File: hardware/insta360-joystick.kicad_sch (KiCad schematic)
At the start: 12 parts

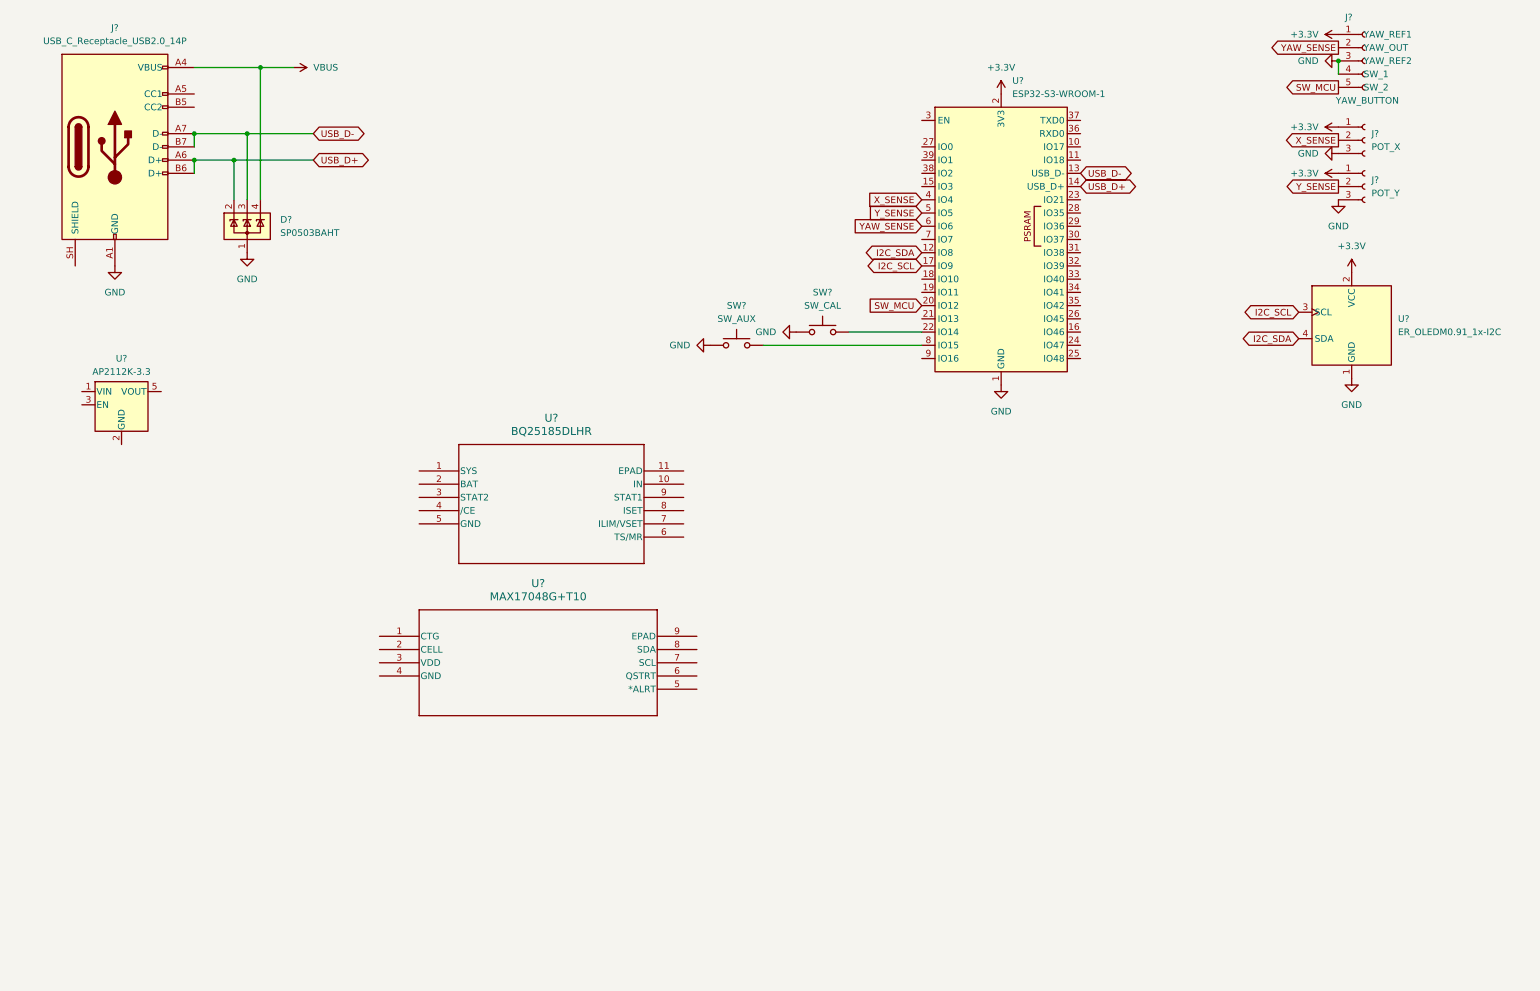
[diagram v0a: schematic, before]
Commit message: Ok I think the schematic is done?
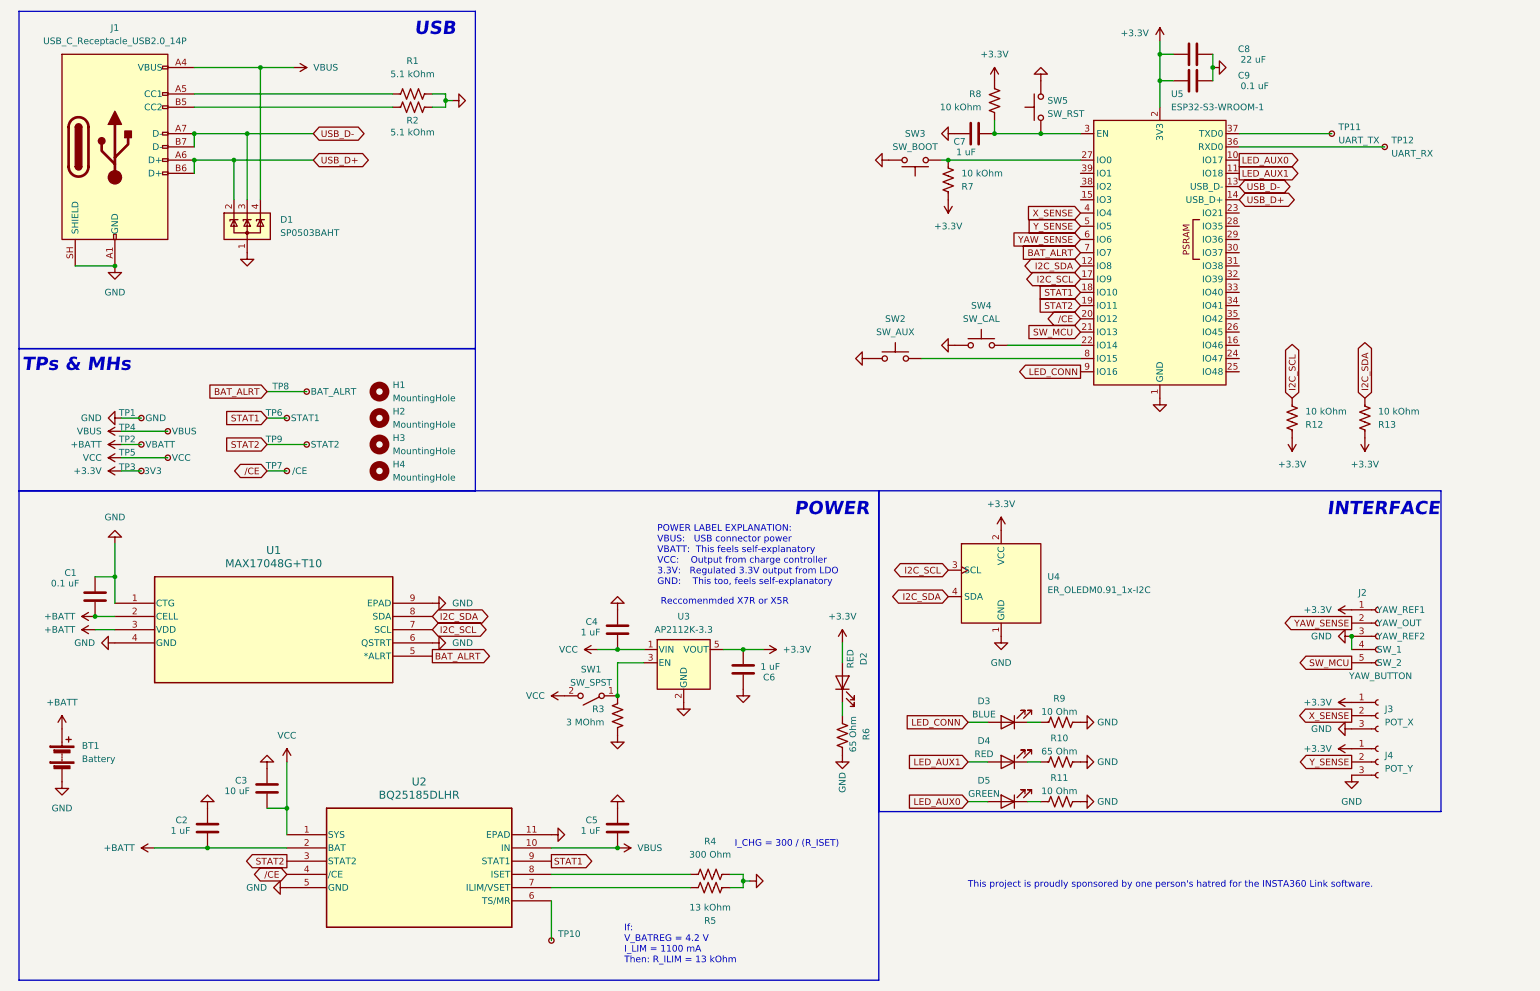
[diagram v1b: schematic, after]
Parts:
- removed U?: AP2112K-3.3, Package_TO_SOT_SMD:SOT-23-5, symbol Regulator_Linear:AP2112K-3.3
- added BT1: Battery, symbol Device:Battery
- added C1, C9: 0.1 uF, symbol Device:C
- added C2, C4, C5, C6, C7: 1 uF, symbol Device:C
- added C3: 10 uF, symbol Device:C
- added C8: 22 uF, symbol Device:C
- added D2, D4: RED, symbol Device:LED
- added D3: BLUE, symbol Device:LED
- added D5: GREEN, symbol Device:LED
- added H1, H2, H3, H4: MountingHole, MountingHole:MountingHole_2.2mm_M2_Pad_TopBottom, symbol Mechanical:MountingHole
- added R1, R2: 5.1 kOhm, symbol Device:R_US
- added R10, R6: 65 Ohm, symbol Device:R_US
- added R11, R9: 10 Ohm, symbol Device:R_US
- added R12, R13, R7, R8: 10 kOhm, symbol Device:R_US
- added R3: 3 MOhm, symbol Device:R_US
- added R4: 300 Ohm, symbol Device:R_US
- added R5: 13 kOhm, symbol Device:R_US
- added SW1: SW_SPST, symbol Switch:SW_SPST
- added SW3: SW_BOOT, symbol Switch:SW_Push
- added SW5: SW_RST, symbol Switch:SW_Push
- added TP1: GND, TestPoint:TestPoint_THTPad_D2.0mm_Drill1.0mm, symbol Connector:TestPoint_Small
- added TP10: TestPoint_Small, TestPoint:TestPoint_Bridge_Pitch2.0mm_Drill0.7mm, symbol Connector:TestPoint_Small
- added TP11: UART_TX, TestPoint:TestPoint_THTPad_D2.0mm_Drill1.0mm, symbol Connector:TestPoint_Small
- added TP12: UART_RX, TestPoint:TestPoint_THTPad_D2.0mm_Drill1.0mm, symbol Connector:TestPoint_Small
- added TP2: VBATT, TestPoint:TestPoint_THTPad_D2.0mm_Drill1.0mm, symbol Connector:TestPoint_Small
- added TP3: 3V3, TestPoint:TestPoint_THTPad_D2.0mm_Drill1.0mm, symbol Connector:TestPoint_Small
- added TP4: VBUS, TestPoint:TestPoint_THTPad_D2.0mm_Drill1.0mm, symbol Connector:TestPoint_Small
- added TP5: VCC, TestPoint:TestPoint_THTPad_D2.0mm_Drill1.0mm, symbol Connector:TestPoint_Small
- added TP6: STAT1, TestPoint:TestPoint_THTPad_D2.0mm_Drill1.0mm, symbol Connector:TestPoint_Small
- added TP7: /CE, TestPoint:TestPoint_THTPad_D2.0mm_Drill1.0mm, symbol Connector:TestPoint_Small
- added TP8: BAT_ALRT, TestPoint:TestPoint_THTPad_D2.0mm_Drill1.0mm, symbol Connector:TestPoint_Small
- added TP9: STAT2, TestPoint:TestPoint_THTPad_D2.0mm_Drill1.0mm, symbol Connector:TestPoint_Small
- added U3: AP2112K-3.3, Package_TO_SOT_SMD:SOT-23-5, symbol Regulator_Linear:AP2112K-3.3
- gave numbers to parts that had none: 11
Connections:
- net +3.3V: now also C6.2, C8.2, C9.2, D2.2 (A), R12.1, R13.1, R7.1, R8.1, TP3.1, U3.5 (VOUT)
- net GND: now also J1.SH (SHIELD), U1.1 (CTG), U1.4 (GND), U1.6 (QSTRT), U1.9 (EPAD), U2.11 (EPAD), U2.5 (GND), BT1.2 (-), C1.1, C2.1, C3.1, C4.1, C5.1, C6.1, C7.1, C8.1, C9.1, R1.2, R10.2, R11.2, R2.2, R3.1, R4.2, R5.2, R6.2, R9.2, SW3.1, SW5.2, TP1.1, U3.2 (GND)
- net I2C_SCL: now also U1.7 (SCL), R12.2
- net I2C_SDA: now also U1.8 (SDA), R13.2
- net SW_MCU: now also U5.21 (IO13); no longer U5.20 (IO12)
- net VBUS: now also U2.10 (IN), C5.2, TP4.1
- net VCC: now reaches U2.1 (SYS)
- net VCC: now also C3.2, C4.2, SW1.2 (B), TP5.1, U3.1 (VIN)
- net +BATT: now reaches U2.2 (BAT)
- net +BATT: now also U1.2 (CELL), U1.3 (VDD), BT1.1 (+), C1.2, C2.2, TP2.1
- net STAT2: now reaches U2.3 (STAT2)
- net STAT2: now also U5.19 (IO11), TP9.1
- net /CE: now reaches U2.4 (/CE)
- net /CE: now also U5.20 (IO12), TP7.1
- net at U2.6 (TS/MR): now also TP10.1
- net at U2.7 (ILIM/VSET): now also R5.1
- net at U2.8 (ISET): now also R4.1
- net STAT1: now reaches U2.9 (STAT1)
- net STAT1: now also U5.18 (IO10), TP6.1
- net BAT_ALRT: now reaches U1.5 (*ALRT)
- net BAT_ALRT: now also U5.7 (IO7), TP8.1
- net at J1.A5 (CC1): now also R1.1
- net at J1.B5 (CC2): now also R2.1
- net LED_AUX0: now reaches U5.10 (IO17)
- net LED_AUX0: now also D5.2 (A)
- net LED_AUX1: now reaches U5.11 (IO18)
- net LED_AUX1: now also D4.2 (A)
- net at U5.27 (IO0): now also R7.2, SW3.2
- net at U5.3 (EN): now also C7.2, R8.2, SW5.1
- net at U5.36 (RXD0): now also TP12.1
- net at U5.37 (TXD0): now also TP11.1
- net LED_CONN: now reaches U5.9 (IO16)
- net LED_CONN: now also D3.2 (A)
- new net: R3.2, SW1.1 (A), U3.3 (EN)
- new net: D5.1 (K), R11.1
- new net: D4.1 (K), R10.1
- new net: D3.1 (K), R9.1
- new net: D2.1 (K), R6.1
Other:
- note added: "INTERFACE"
- note added: "I_CHG = 300 / (R_ISET)"
- note added: "If: V_BATREG = 4.2 V I_LIM = 1100 mA Then: R_ILIM = 13 kOhm"
- note added: "POWER"
- note added: "POWER LABEL EXPLANATION: VBUS: USB connector power VBATT: This feels self-explanatory VCC: Output from charge controller 3.3V: Regulated 3.3V output from LDO GND: This too, feels self-explanatory"
- note added: "Reccomenmded X7R or X5R"
- note added: "TPs & MHs"
- note added: "This project is proudly sponsored by one person's hatred for the INSTA360 Link software."
- note added: "USB"
- moved on the sheet: J2, J3, J4, SW2, SW4, U4, U5
